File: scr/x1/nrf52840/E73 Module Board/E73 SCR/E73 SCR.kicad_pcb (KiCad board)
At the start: 2 copper layers, 39.4 x 29.7 mm, 29 parts, among them J1 USB_B_Micro, J2 BAT, J3 SWD, J4 EXP, J5 SWTCH, J6 JOY, Q1 AO3401, U1 AP2112K-3.3, U2 MCP73831-2-OT, U3 E73-2G4M08S1C-52840, Y1 32,767 Hz

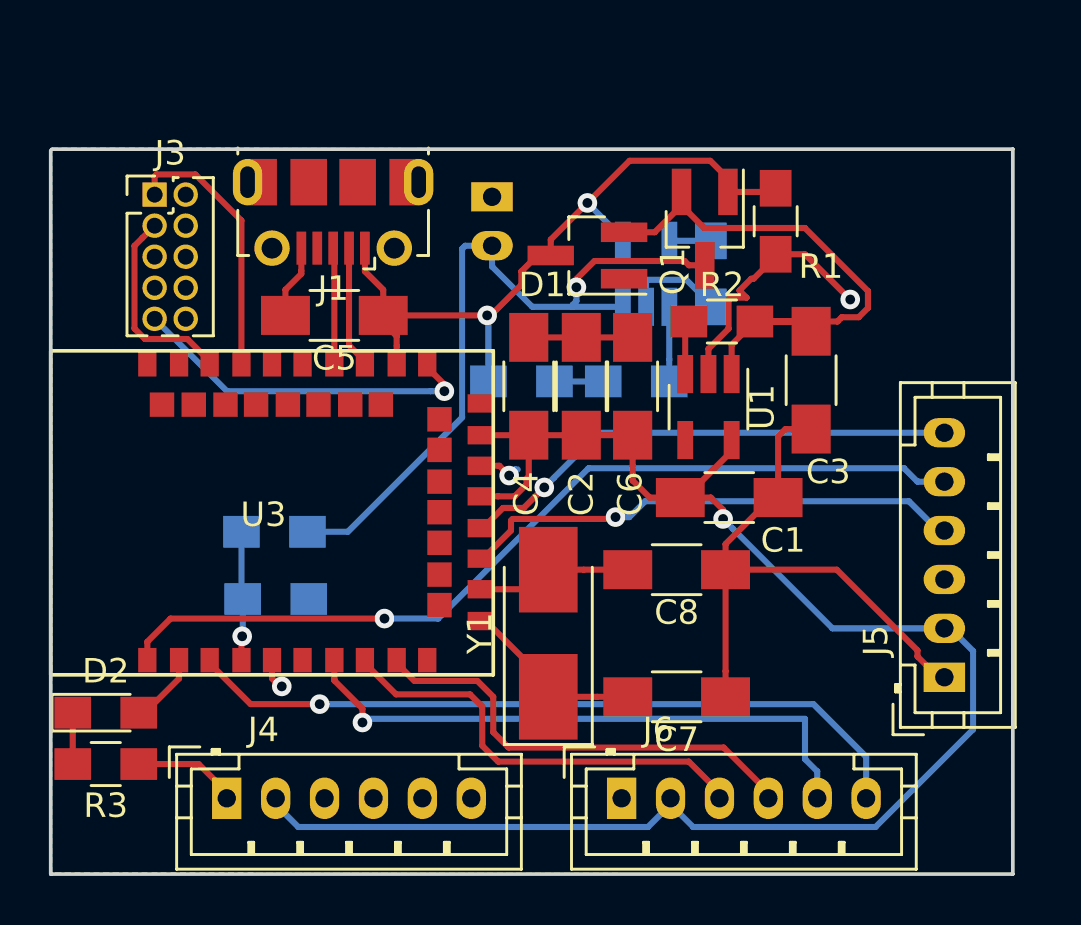
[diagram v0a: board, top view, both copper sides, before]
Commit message: PCB v1.0
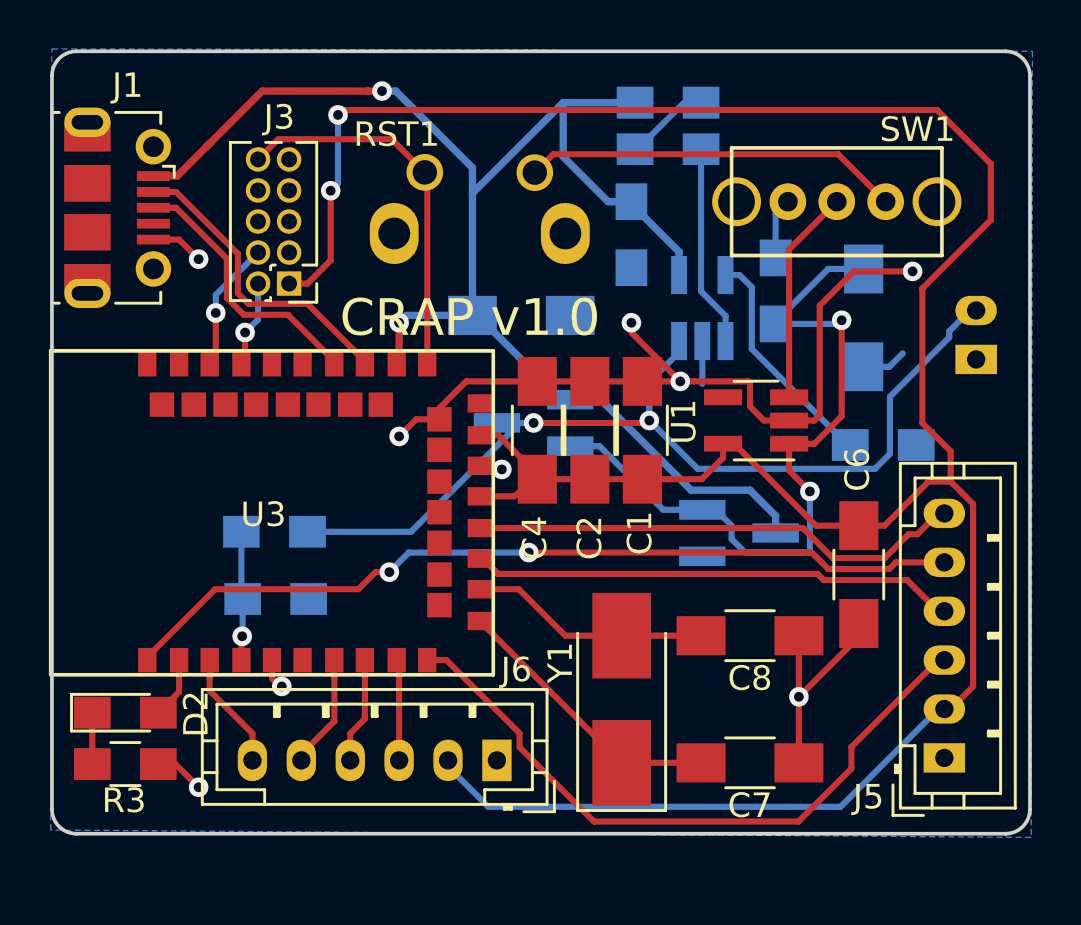
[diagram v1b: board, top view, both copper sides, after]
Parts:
- removed J4: EXP, Connectors_JST:JST_PH_B6B-PH-K_06x2.00mm_Straight
- added RST1: SW_SPST, Switches:Tac_SPST_RightAngle_SideActuated_THT, F.Cu at (129.5, 64.2)
- added SW1: SW_BAT, Switches:OS102011MA1QN1, F.Cu at (144.1, 64.2)
- C3, C5, D1, Q1, R1, R2: moved to B.Cu
- moved J2 20.9 mm to (149.8, 70.6), turned to 90 degrees
- moved D1 12.9 mm to (140.1, 77.7), turned to 0 degrees
- moved D3 12.9 mm to (137.2, 60.1)
- moved C6 12.0 mm to (145.0, 79.4), turned to 270 degrees
- moved Q1 10.6 mm to (131.7, 73.2), turned to 180 degrees
- moved RPROG1 9.93 mm to (146.0, 74.1), turned to 0 degrees
- moved J1 9.73 mm to (113.8, 64.4), turned to 270 degrees
- moved R4 9.59 mm to (137.2, 62.0)
- moved C5 7.65 mm to (131.2, 68.8), turned to 0 degrees
- moved J3 6.60 mm to (121.7, 67.5), turned to 180 degrees
- moved R1 5.93 mm to (135.7, 65.5)
- moved J6 5.33 mm to (130.2, 87.0), turned to 180 degrees
- moved C1 4.49 mm to (136.2, 73.5), turned to 90 degrees
- moved C8 4.04 mm to (140.6, 81.9)
- moved Y1 4.04 mm to (135.3, 84.5)
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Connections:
- J3 pad 1: SWDIO -> +3V3
- J3 pad 10: GND -> RESET
- J3 pad 2: +3V3 -> SWDIO
- J3 pad 3: SWCLK -> GND
- J3 pad 4: GND -> SWCLK
- J3 pad 5: Net-(J3-Pad5) -> GND
- J3 pad 6: GND -> Net-(J3-Pad6)
- J3 pad 8: GND -> Net-(J3-Pad8)
- J3 pad 9: RESET -> GND
- U1 pad 3: Net-(R2-Pad2) -> Net-(SW1-Pad2)
- U3 pad 33: P1_13 -> Net-(U3-Pad33)
- U3 pad 35: P0_24 -> Net-(U3-Pad35)
- U3 pad 41: P0_09 -> Net-(U3-Pad41)
- U3 pad 43: P0_10 -> Net-(U3-Pad43)
- U3 pad 8: X -> Y
- U3 pad 9: Y -> X
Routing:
- net +3V3: track 67.7 -> 109.4 mm, vias 1 -> 2
- net VBUS: track 30.6 -> 61.2 mm
- net LCLK: track 0.00 -> 27.5 mm
- net A1_P003: track 30.3 -> 4.82 mm, vias 1 -> 0
- net SW: track 24.6 -> 4.66 mm, vias 1 -> 0
- net Y: track 18.6 -> 4.47 mm
- net X: track 18.0 -> 4.14 mm
- net GND: track 53.6 -> 66.6 mm, vias 3 -> 10
- net Net-(SW1-Pad2): track 0.00 -> 8.81 mm
- net +BATT: track 30.1 -> 38.0 mm, vias 1 -> 2
- net Net-(RPROG1-Pad1): track 1.70 -> 9.46 mm
- net Net-(C3-Pad1): track 23.0 -> 30.6 mm, vias 0 -> 2
- net D-: track 5.02 -> 12.6 mm
- net SWDIO: track 11.0 -> 3.58 mm, vias 0 -> 1
- net D+: track 4.77 -> 11.1 mm
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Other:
- board size 39.4 x 29.7 mm -> 40 x 32 mm
- net class VBUS added: clearance 0.25, trace_width 0.3, via_dia 0.8, via_drill 0.4
- board text added: "CRAP v1.0"
- board text added: "CRAP v1.0 2019-04 For Shane Thomson By Ben Von Handorf"
